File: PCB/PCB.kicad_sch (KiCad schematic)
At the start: 28 parts, among them J1 USB_C_Receptacle_USB2.0_16P, U1 HT-CT62, U2 SAM-M10Q, U3 ER_OLEDM0.91_1x-I2C, U4 TPS63001, U5 TPS22917DBV, U6 BQ24074RGT

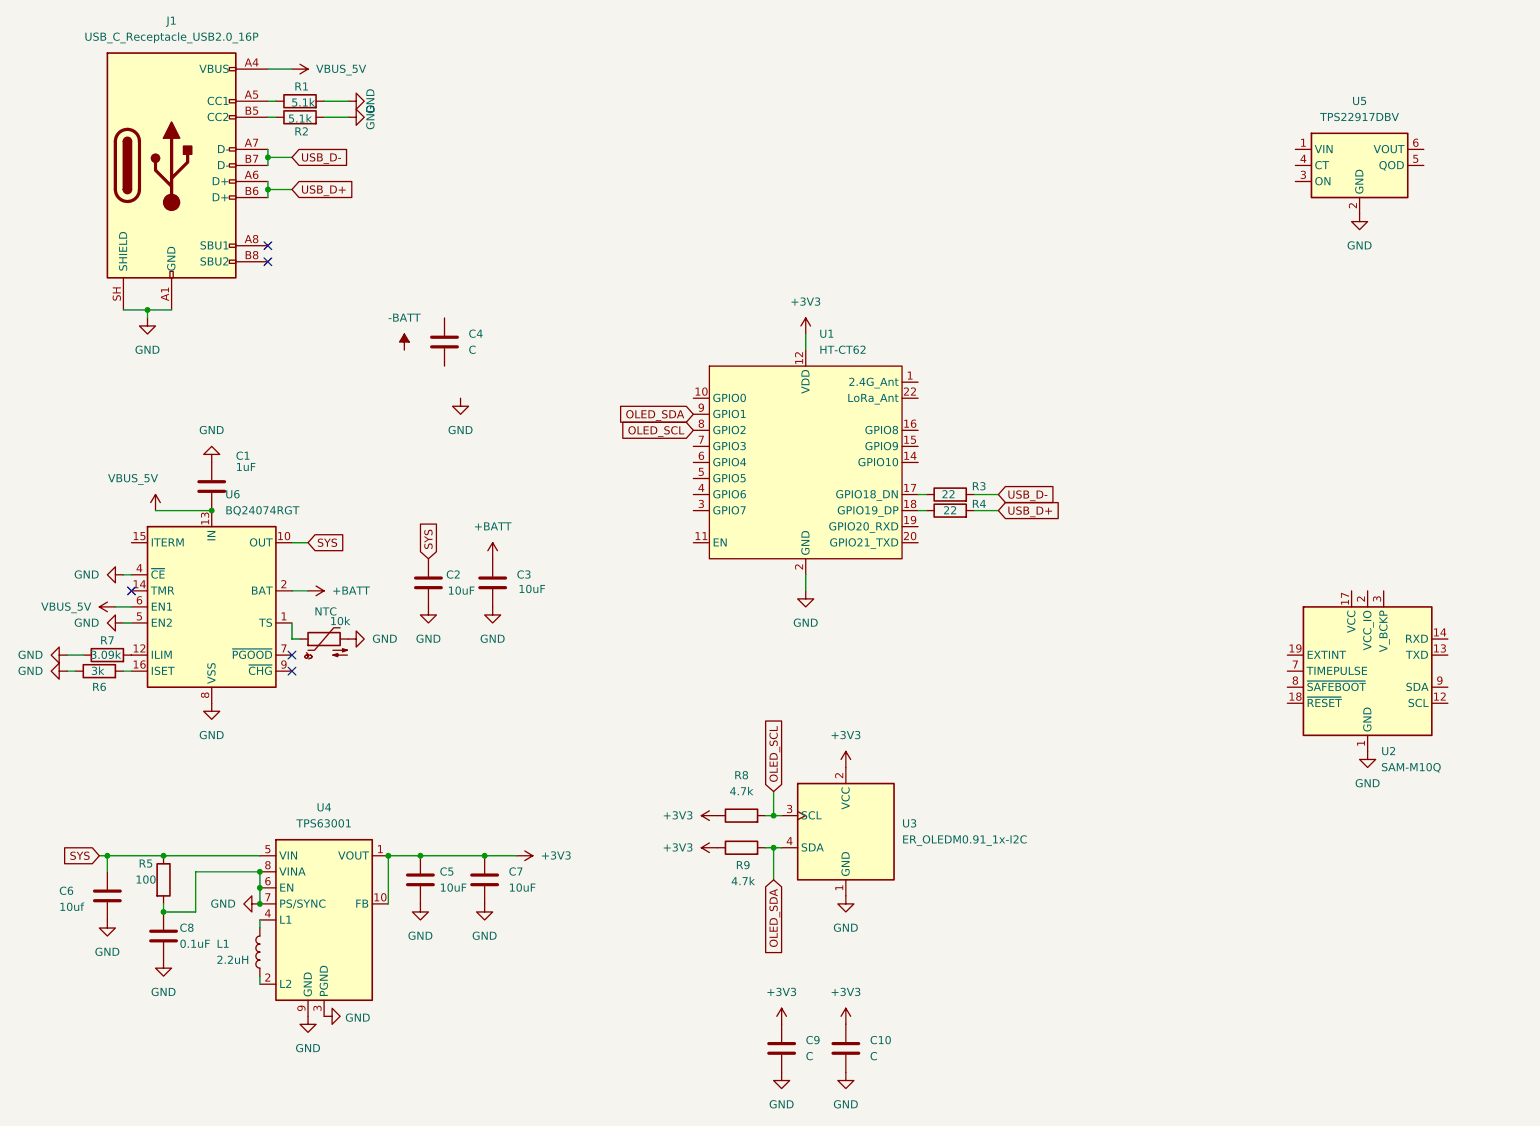
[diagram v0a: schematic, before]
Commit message: mapped the ht-ct62
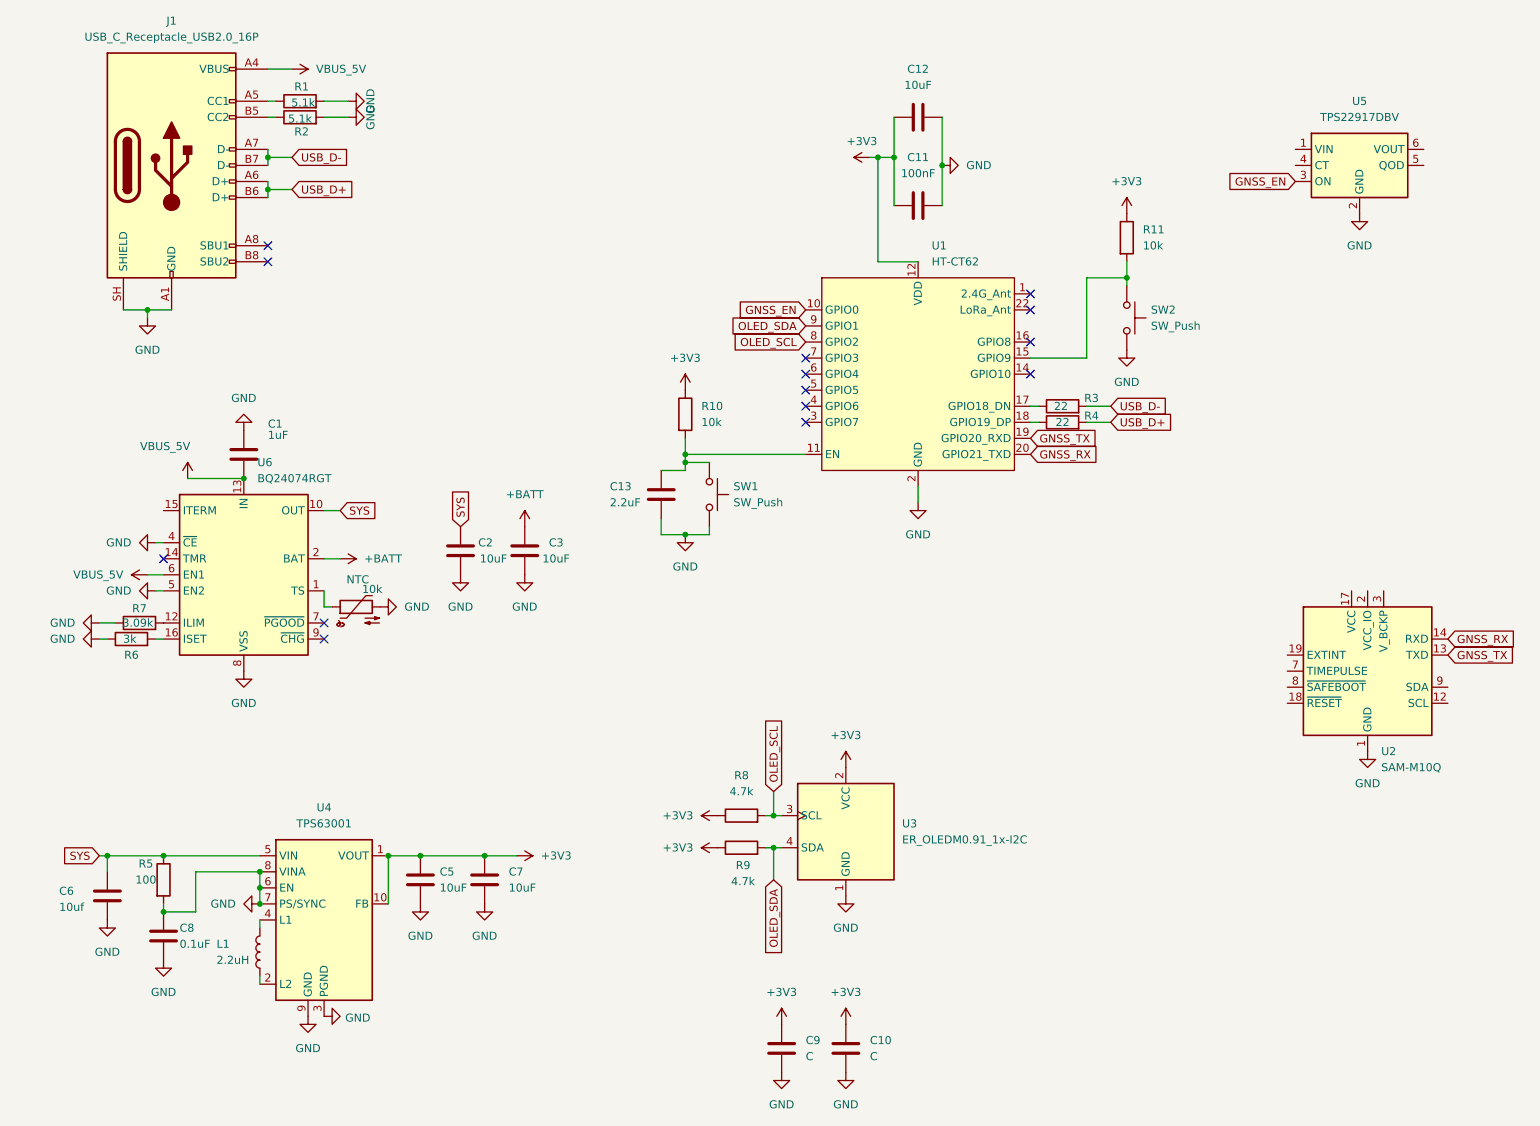
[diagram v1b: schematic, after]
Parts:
- removed C4: C, symbol Device:C
- added C11: 100nF, symbol Device:C
- added C12: 10uF, symbol Device:C
- added C13: 2.2uF, symbol Device:C
- added R10, R11: 10k, symbol Device:R
- added SW1, SW2: SW_Push, symbol Switch:SW_Push
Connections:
- net +3V3: now also C11.2, C12.2, R10.1, R11.1
- net GND: now also C11.1, C12.1, C13.2, SW1.2, SW2.2
- net GNSS_EN: now reaches U5.3 (ON)
- net GNSS_EN: now also U1.10 (GPIO0)
- net GNSS_TX: now reaches U2.13 (TXD)
- net GNSS_TX: now also U1.19 (GPIO20_RXD)
- net GNSS_RX: now reaches U2.14 (RXD)
- net GNSS_RX: now also U1.20 (GPIO21_TXD)
- net at U1.11 (EN): now also C13.1, R10.2, SW1.1
- net at U1.15 (GPIO9): now also R11.2, SW2.1
- no-connect marks 5 -> 14
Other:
- moved on the sheet: C1, C2, C3, NTC, R3, R4, R6, R7, U1, U6
